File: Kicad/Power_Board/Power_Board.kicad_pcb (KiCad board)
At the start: 2 copper layers, 40.6 x 14 mm, 18 parts, among them J1 Conn_01x04_Pin, J2 Screw_Terminal_01x02, U1 PTPS543021DRLR, U2 PTPS543021DRLR

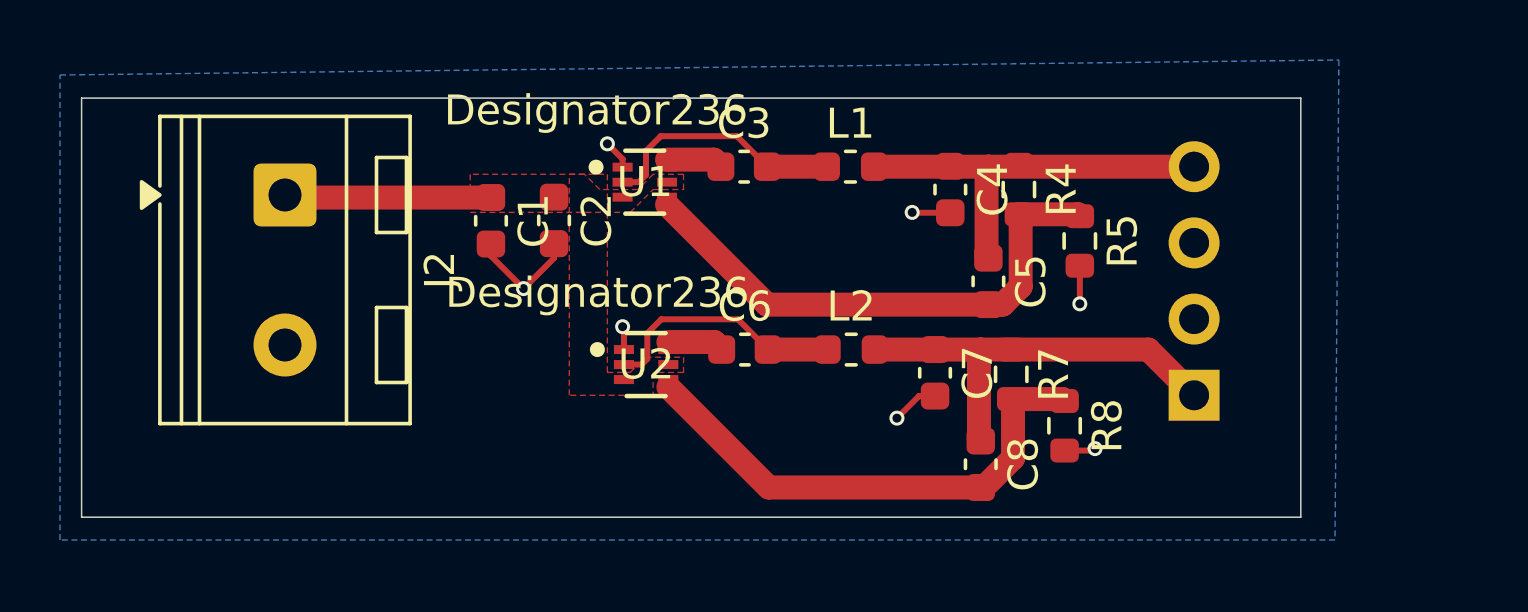
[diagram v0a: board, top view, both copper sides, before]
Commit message: Wrote v1 of the code, final version of boards
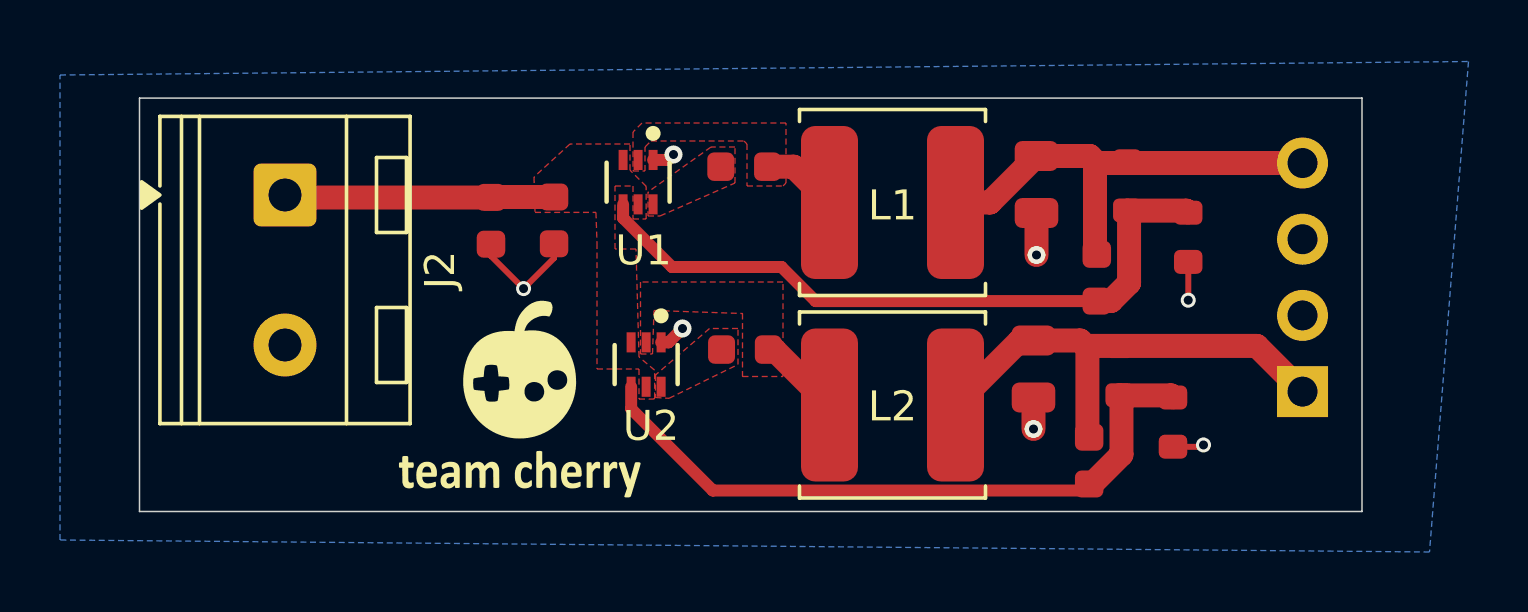
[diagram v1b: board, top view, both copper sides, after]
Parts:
- added G***: LOGO, LOGO, F.Cu at (60.3, 74.8)
- C1: value 10u -> 10uF; footprint Capacitor_SMD:C_0603_1608Metric -> PCM_JLCPCB:C_0603
- C2, C3, C6: value 0.1u -> 100nF; footprint Capacitor_SMD:C_0603_1608Metric -> PCM_JLCPCB:C_0603
- C4: value 44u -> 47uF; footprint Capacitor_SMD:C_0603_1608Metric -> PCM_JLCPCB:C_0805
- C5: value 75p -> 68pF; footprint Capacitor_SMD:C_0603_1608Metric -> PCM_JLCPCB:C_0603
- C7: value 60u -> 22uF; footprint Capacitor_SMD:C_0603_1608Metric -> PCM_JLCPCB:C_0805
- C8: value 100p -> 100pF; footprint Capacitor_SMD:C_0603_1608Metric -> PCM_JLCPCB:C_0603
- L1: footprint Inductor_SMD:L_0603_1608Metric -> Inductor_SMD:L_TDK_VLS6045EX_VLS6045AF
- L2: value 5uH -> 4.7uH; footprint Inductor_SMD:L_0603_1608Metric -> Inductor_SMD:L_TDK_VLS6045EX_VLS6045AF
- R4, R7: value 100k -> 100kΩ; footprint Resistor_SMD:R_0603_1608Metric -> PCM_JLCPCB:R_0603
- R5: value 22.1k -> 22kΩ; footprint Resistor_SMD:R_0603_1608Metric -> PCM_JLCPCB:R_0603
- R8: value 5.25k -> 5.1kΩ; footprint Resistor_SMD:R_0603_1608Metric -> PCM_JLCPCB:R_0603
- moved C5 3.62 mm to (79.6, 70.8)
- moved C8 3.62 mm to (79.3, 76.9)
- moved J1 3.62 mm to (86.4, 74.6)
- moved R5 3.62 mm to (82.6, 69.4)
- moved R7 3.62 mm to (80.3, 73.9)
- moved R4 3.62 mm to (80.6, 67.7)
- moved R8 3.62 mm to (82.1, 75.6)
- moved C7 3.28 mm to (77.5, 73.8)
- moved C4 2.88 mm to (77.5, 67.7)
- moved L2 2.30 mm to (72.8, 75.0)
- moved L1 1.84 mm to (72.8, 68.2)
- moved U1 0.22 mm to (64.3, 67.6), turned to -90 degrees
- turned U2 to -90 degrees
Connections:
- net Net-(U1-FB) renamed /FB
- net Net-(U2-BOOT) renamed /BOOT 12V
- net Net-(U2-FB) renamed /FB 12V
- net Net-(U2-SW) renamed /SW 12V
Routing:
- net /SW: track 8.33 -> 2.56 mm
- net /SW 12V: track 8.33 -> 2.80 mm
- net /FB 12V: track 17.1 -> 22.5 mm
- net /FB: track 17.9 -> 23.2 mm
- net /20V VIN: track 6.90 -> 9.01 mm
- net /Boot: track 1.89 -> 0.00 mm
- net /BOOT 12V: track 1.88 -> 0.00 mm
- net /12v Output: track 14.4 -> 16.2 mm
- net /3v3 Output: track 13.8 -> 15.4 mm
- added copper zone on F.Cu, net /BOOT 12V
- added copper zone on F.Cu, net /Boot
- added copper zone on F.Cu, net /SW
- added copper zone on F.Cu, net /SW 12V
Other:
- board size 40.6 x 14 mm -> 40.8 x 13.8 mm
